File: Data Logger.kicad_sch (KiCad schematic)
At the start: 25 parts, among them U1 24LC1025, U2 DS1339U-3+, U3 24LC1025, U4 ATMEGA328P-AU, Y1 32 KHz, Y2 16 MHz

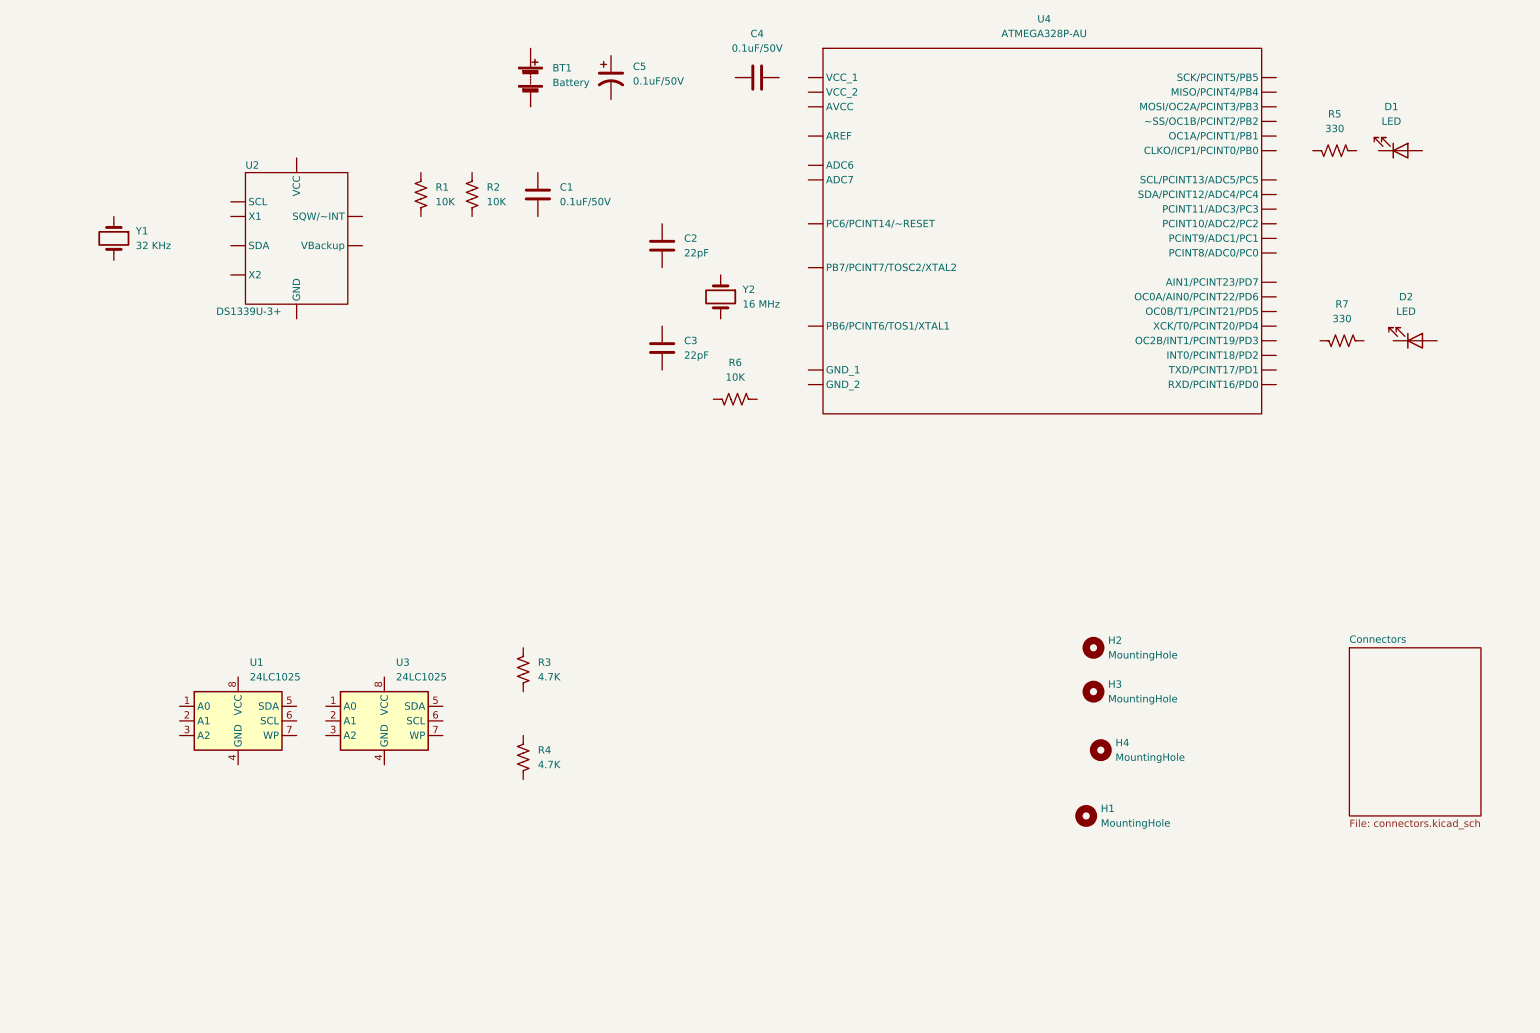
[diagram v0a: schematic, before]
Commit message: update schematics
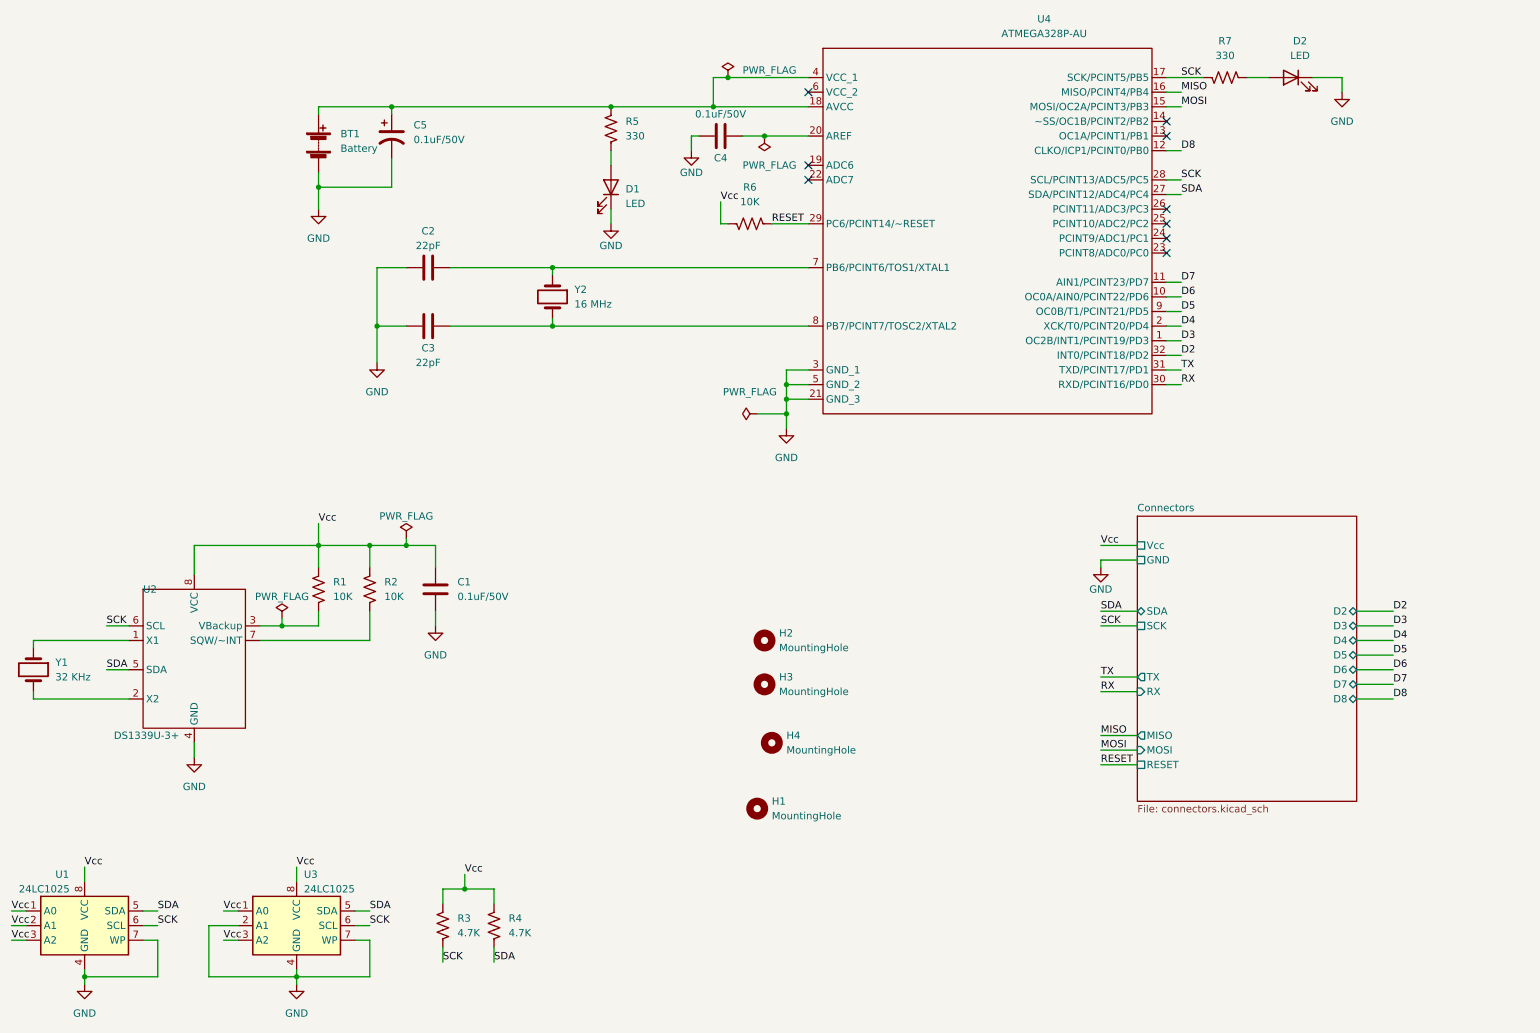
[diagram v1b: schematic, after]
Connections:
- net GND: now reaches D2.1 (K)
- net GND: now also BT1.2 (-), C1.2, C2.2, C3.1, C4.2, C5.2, D1.1 (K), U1.4 (GND), U1.7 (WP), U2.4 (GND), U3.2 (A1), U3.4 (GND), U3.7 (WP), U4.21 (GND_3), U4.3 (GND_1), U4.5 (GND_2)
- net at D2.2 (A): now also R7.1
- net Vcc: now reaches R3.1
- net Vcc: now also C1.1, R1.2, R2.2, R4.1, R6.2, U1.1 (A0), U1.2 (A1), U1.3 (A2), U1.8 (VCC), U2.8 (VCC), U3.1 (A0), U3.3 (A2), U3.8 (VCC)
- net SCK: now reaches R3.2
- net SCK: now also R7.2, U1.6 (SCL), U2.6 (SCL), U3.6 (SCL), U4.17 (SCK/PCINT5/PB5), U4.28 (SCL/PCINT13/ADC5/PC5)
- net SDA: now reaches U1.5 (SDA)
- net SDA: now also R4.2, U2.5 (SDA), U3.5 (SDA), U4.27 (SDA/PCINT12/ADC4/PC4)
- net at C5.1: now also BT1.1 (+), R5.2, U4.18 (AVCC), U4.4 (VCC_1)
- net RESET: now reaches R6.1
- net RESET: now also U4.29 (PC6/PCINT14/~RESET)
- net at Y2.1: now also C2.1, U4.7 (PB6/PCINT6/TOS1/XTAL1)
- net at Y2.2: now also C3.2, U4.8 (PB7/PCINT7/TOSC2/XTAL2)
- net at Y1.1: now also U2.1 (X1)
- net at Y1.2: now also U2.2 (X2)
- net at R1.1: now also U2.3 (VBackup)
- net at C4.1: now also U4.20 (AREF)
- net at R2.1: now also U2.7 (SQW/~INT)
- net at R5.1: now also D1.2 (A)
- new net D2: U4.32 (INT0/PCINT18/PD2)
- new net D3: U4.1 (OC2B/INT1/PCINT19/PD3)
- new net D4: U4.2 (XCK/T0/PCINT20/PD4)
- new net D5: U4.9 (OC0B/T1/PCINT21/PD5)
- new net D6: U4.10 (OC0A/AIN0/PCINT22/PD6)
- new net D7: U4.11 (AIN1/PCINT23/PD7)
- new net D8: U4.12 (CLKO/ICP1/PCINT0/PB0)
- new net MISO: U4.16 (MISO/PCINT4/PB4)
- new net MOSI: U4.15 (MOSI/OC2A/PCINT3/PB3)
- new net RX: U4.30 (RXD/PCINT16/PD0)
- new net TX: U4.31 (TXD/PCINT17/PD1)
- no-connect marks 0 -> 9
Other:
- sheet Connectors ports: added D2, D3, D4, D5, D6, D7, D8, GND, MISO, MOSI, RESET, RX, SCK, SDA, TX, Vcc; removed none
- moved on the sheet: BT1, C1, C2, C3, C4, C5, D1, D2, H1, H2, H3, H4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

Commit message: Completed Routing
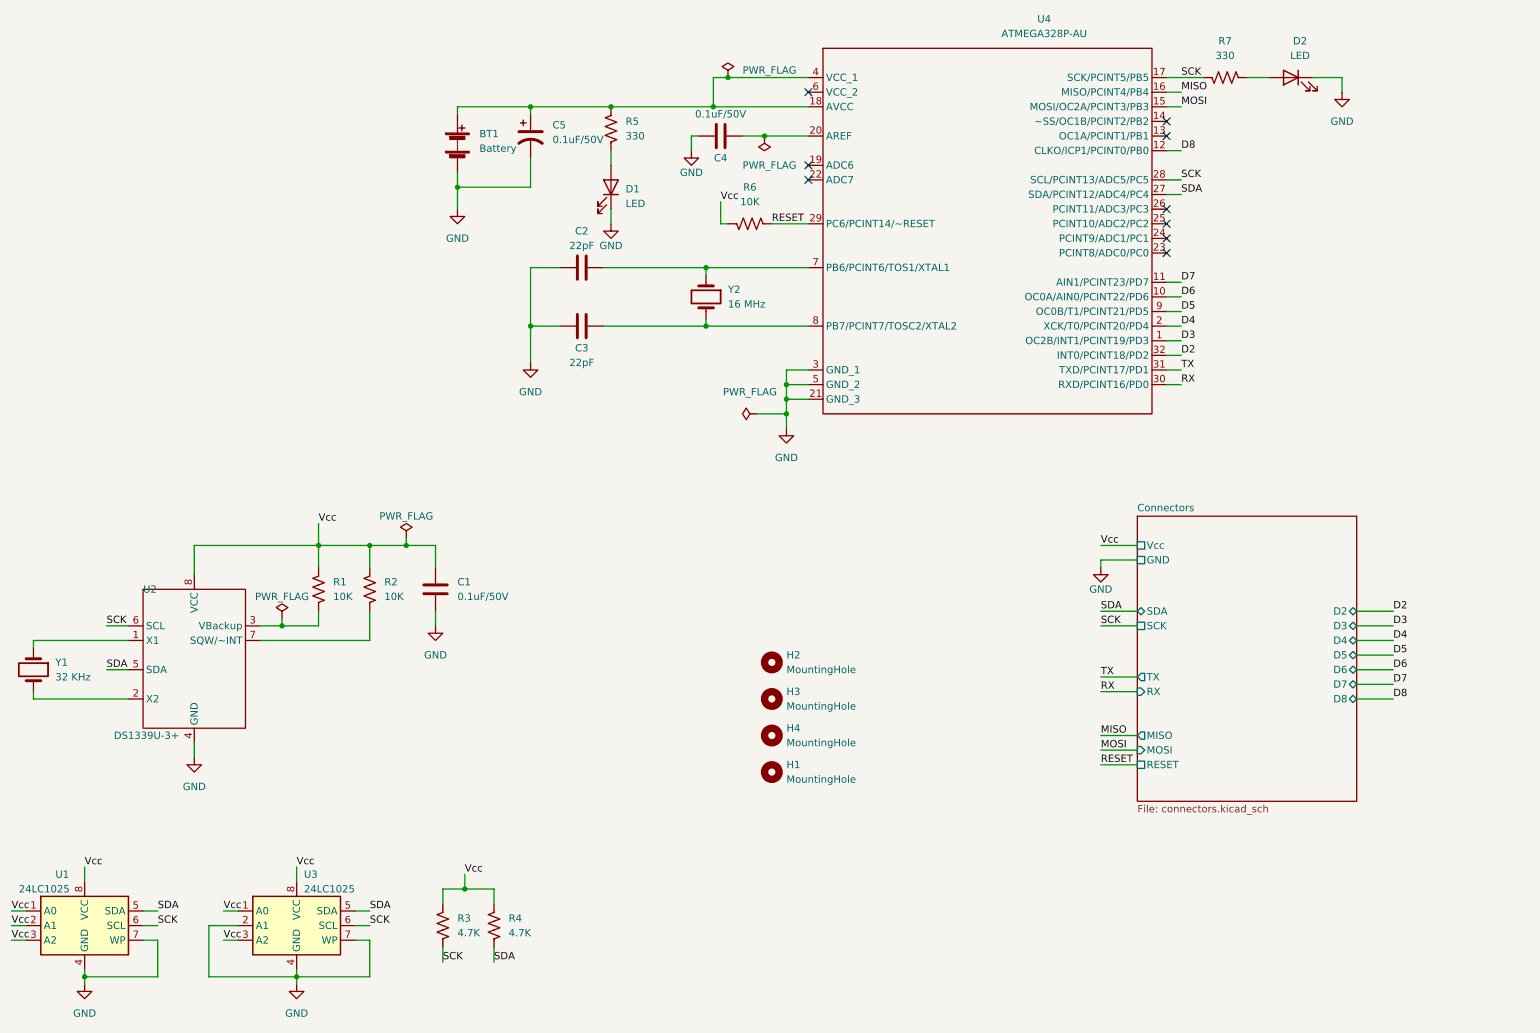
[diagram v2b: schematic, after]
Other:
- moved on the sheet: BT1, C2, C3, C5, H1, H2, H3, H4, Y2
